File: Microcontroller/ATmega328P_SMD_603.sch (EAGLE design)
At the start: 13 parts, among them Q2 16MHz, U1 ATMEGA328P_TQFP

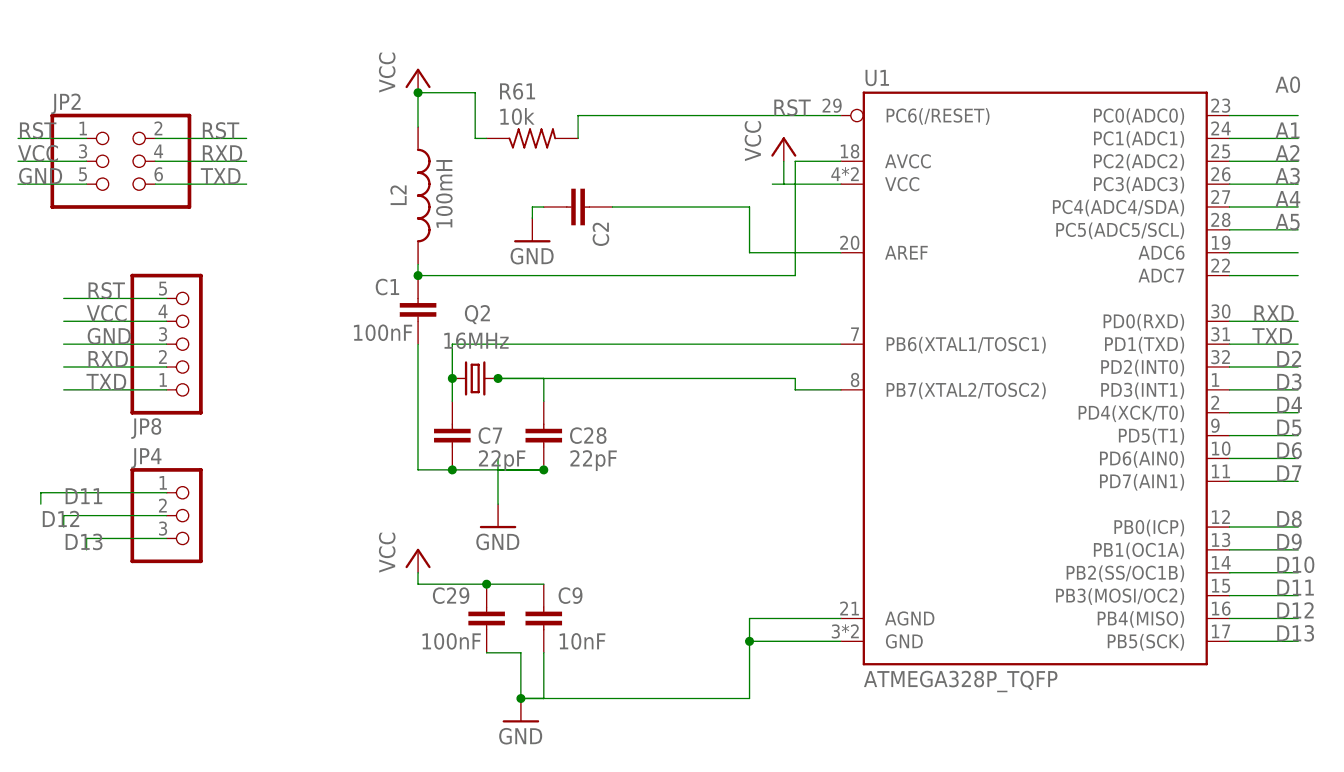
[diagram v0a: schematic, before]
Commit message: updated atmega ckt
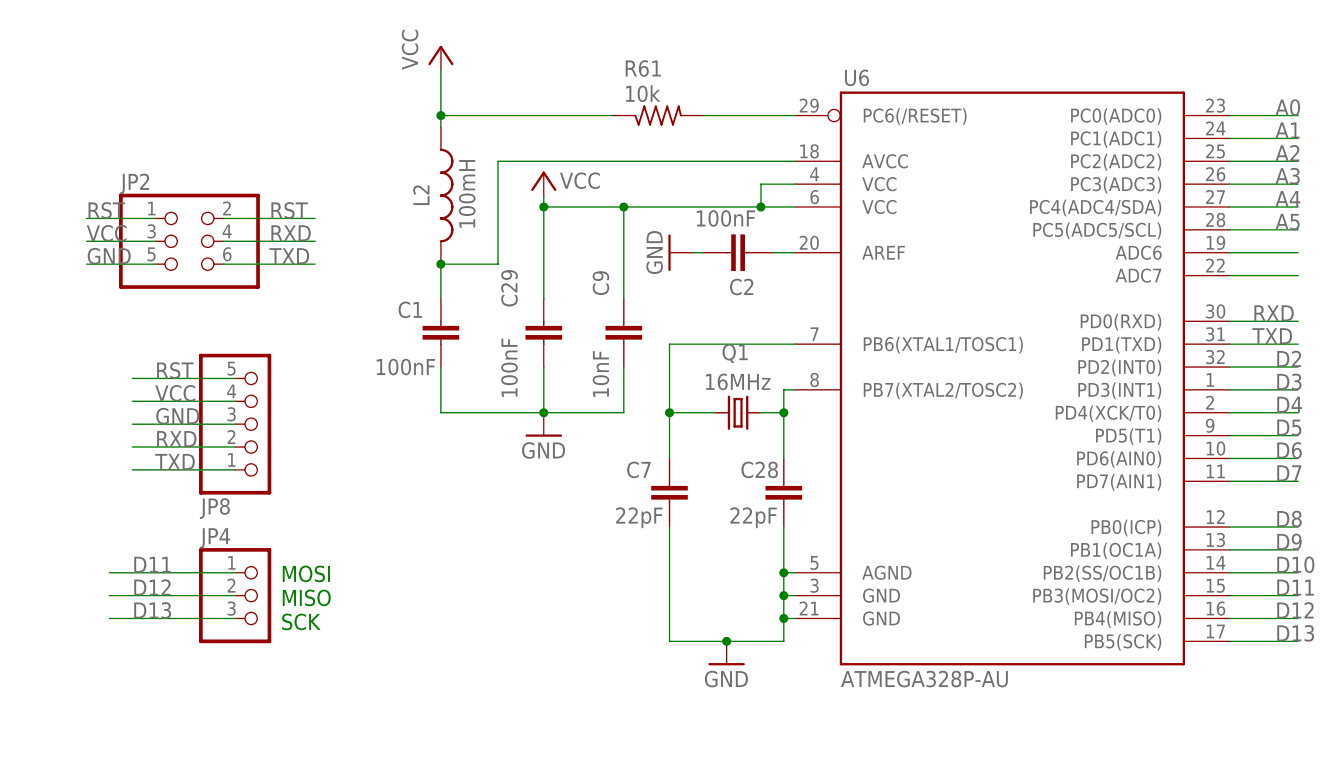
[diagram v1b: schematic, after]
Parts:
- removed Q2: 16MHz, SparkFun-Clocks:CRYSTAL-16MHZSMD-5X3.2
- removed U1: ATMEGA328P_TQFP, SparkFun-IC-Microcontroller:ATMEGA328P_TQFP
- added Q1: 16MHz, crystal-geyer_V1_0:KX-7
- added U6: ATMEGA328P-AU, SparkFun:ATMEGA168
- C2: value (none) -> 100nF
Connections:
- removed net A0: U1.PC0(ADC0)
- removed net A1: U1.PC1(ADC1)
- removed net A2: U1.PC2(ADC2)
- removed net A3: U1.PC3(ADC3)
- removed net A4: U1.PC4(ADC4/SDA)
- removed net A5: U1.PC5(ADC5/SCL)
- removed net D10: U1.PB2(SS/OC1B)
- removed net D2: U1.PD2(INT0)
- removed net D3: U1.PD3(INT1)
- removed net D4: U1.PD4(XCK/T0)
- removed net D5: U1.PD5(T1)
- removed net D6: U1.PD6(AIN0)
- removed net D7: U1.PD7(AIN1)
- removed net D8: U1.PB0(ICP)
- removed net D9: U1.PB1(OC1A)
- removed net N$13: U1.ADC6
- removed net N$14: U1.ADC7
- removed net N$6: C2.1, U1.AREF
- new net N$1: C2.1, U6.AREF
- new net RESET: R61.2, U6.PC6(/RESET)
- net D11: no longer U1.PB3(MOSI/OC2)
- net D12: no longer U1.PB4(MISO)
- net D13: no longer U1.PB5(SCK)
- net GND: now also U6.AGND, U6.GND@1, U6.GND@2; no longer U1.AGND, U1.GND
- net N$2: now also Q1.1, U6.PB7(XTAL2/TOSC2); no longer Q2.1, U1.PB7(XTAL2/TOSC2)
- net N$3: now also Q1.2, U6.PB6(XTAL1/TOSC1); no longer Q2.2, U1.PB6(XTAL1/TOSC1)
- net N$5: now also U6.AVCC; no longer U1.AVCC
- net RST: no longer R61.2, U1.PC6(/RESET)
- net RXD: no longer U1.PD0(RXD)
- net TXD: no longer U1.PD1(TXD)
- net VCC: now also U6.VCC@1, U6.VCC@2; no longer U1.VCC
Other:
- note added: "MOSI MISO SCK"
- moved on the sheet: C1, C2, C28, C29, C7, C9, JP2, JP4, JP8, L2, R61
